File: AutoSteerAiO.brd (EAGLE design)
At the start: 114.3 x 99.1 mm, 81 parts, among them IC2 MMA8452Q, J4 CONNECTOR 1x5 PINS, K4 CB1A-P-12V

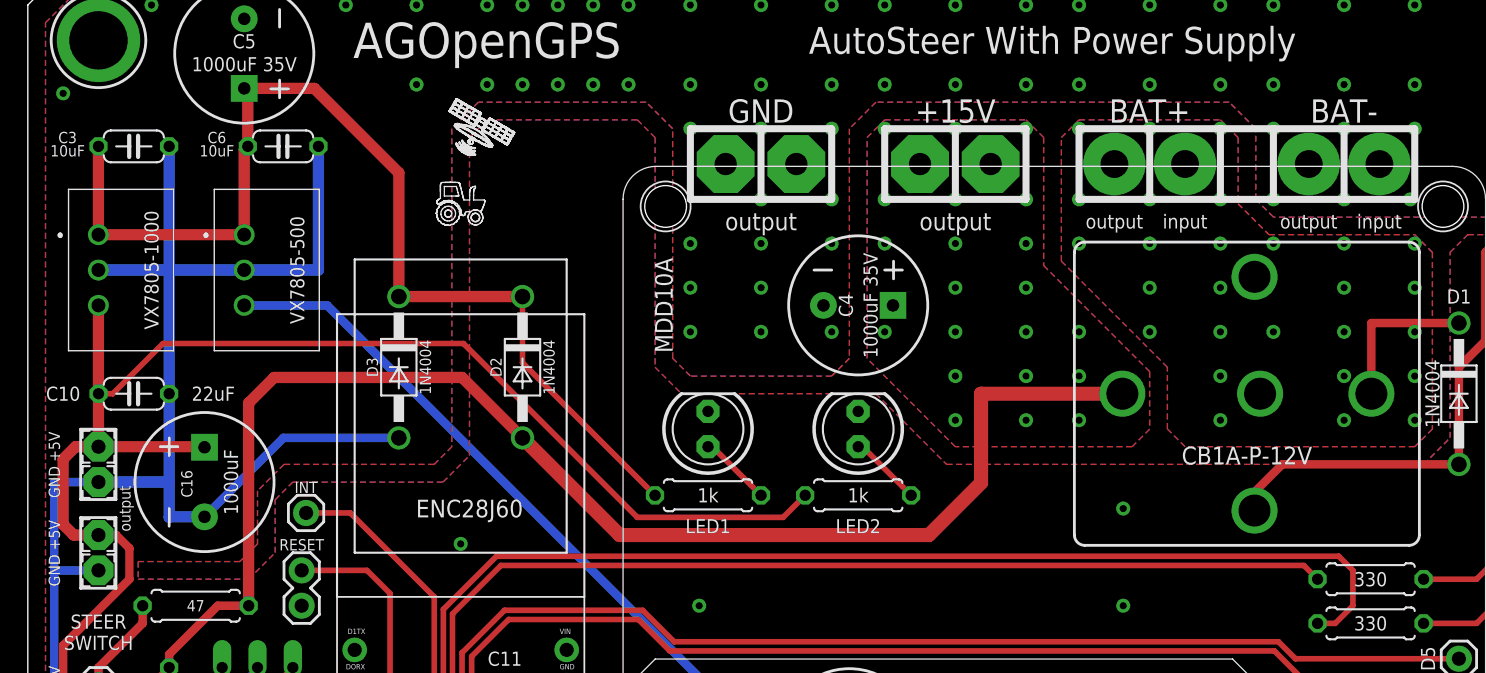
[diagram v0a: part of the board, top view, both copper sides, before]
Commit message: Add files via upload
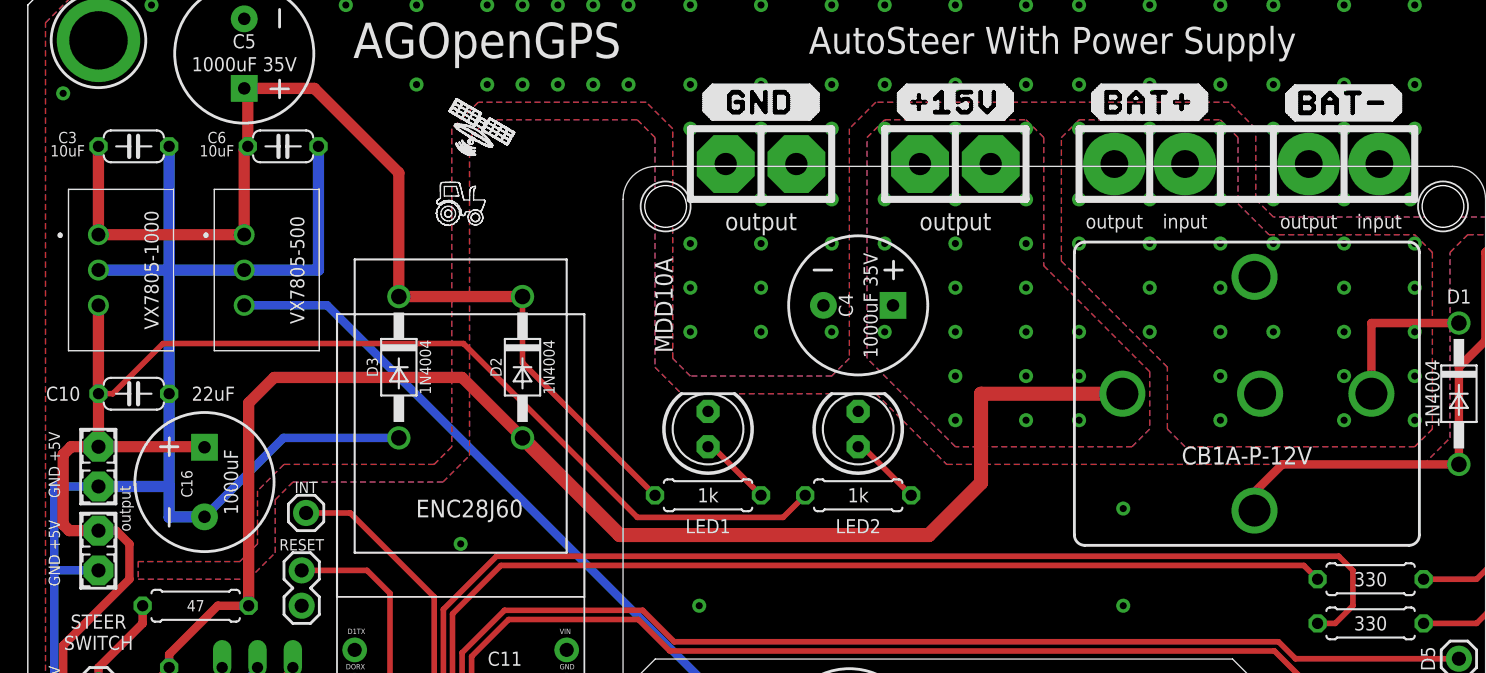
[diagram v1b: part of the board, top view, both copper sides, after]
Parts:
- moved +5V 0.32 mm to (12.7, 79.1)
- moved GND34 0.32 mm to (12.7, 82.2)
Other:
- board text removed: "BAT+"
- board text removed: "BAT-"
